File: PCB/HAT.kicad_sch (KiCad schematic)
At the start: 0 parts

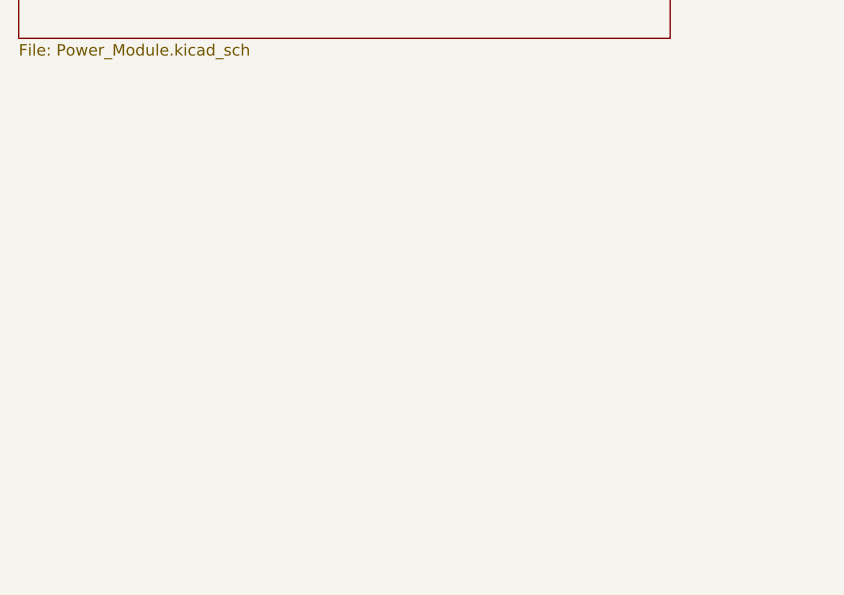
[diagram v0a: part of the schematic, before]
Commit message: Add microcontroller interfacing schematic
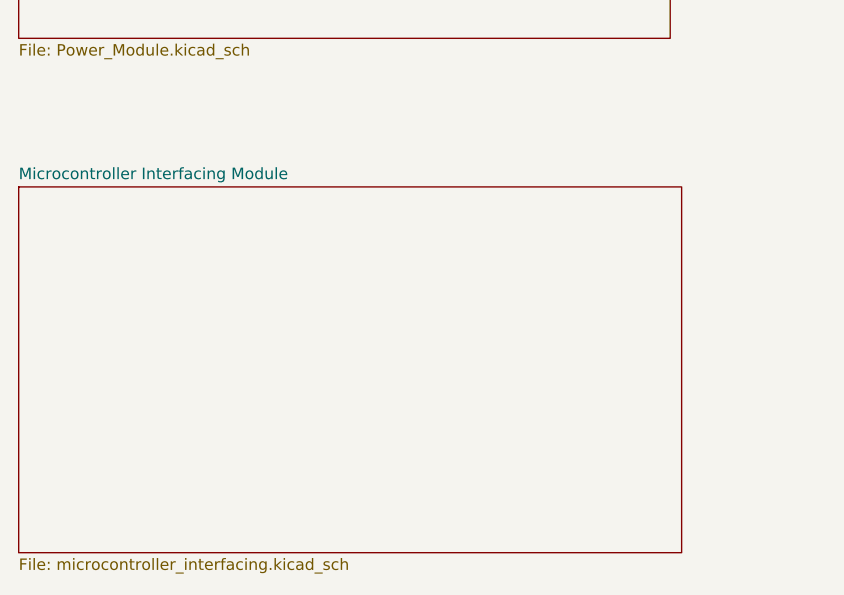
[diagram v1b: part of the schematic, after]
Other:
- added sheet Microcontroller Interfacing Module (microcontroller_interfacing.kicad_sch)
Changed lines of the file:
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@@
+    )
+  )
+  (sheet (at 40.64 83.82) (size 73.66 40.64) (fields_autoplaced)
+    (stroke (width 0.1524) (type solid))
+    (fill (color 0 0 0 0.0000))
+    (property "Sheetname" "Microcontroller Interfacing Module" (at 40.64 83.1084 0)
+      (effects (font (size 1.27 1.27)) (justify left bottom))
+    )
+    (property "Sheetfile" "microcontroller_interfacing.kicad_sch" (at 40.64 125.0446 0)
+      (effects (font (size 1.27 1.27)) (justify left top))
+    )
+    (instances
+      (project "HAT"
+        (path "/40f36b19-a08c-43e7-88a6-ec8387939712" (page "4"))
+      )
     )
   )
